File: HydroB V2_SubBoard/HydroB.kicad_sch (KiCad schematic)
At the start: 0 parts

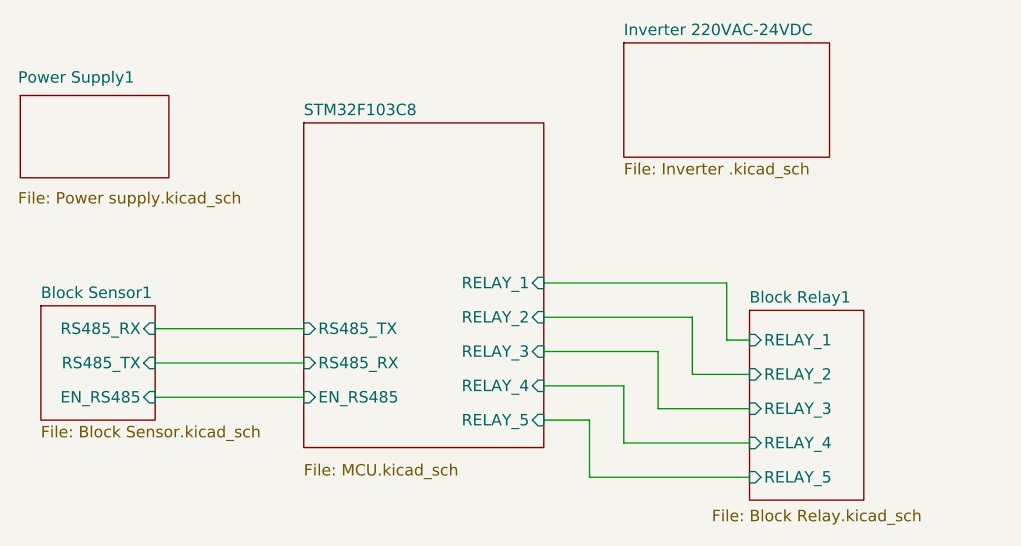
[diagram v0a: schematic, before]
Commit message: PCB update
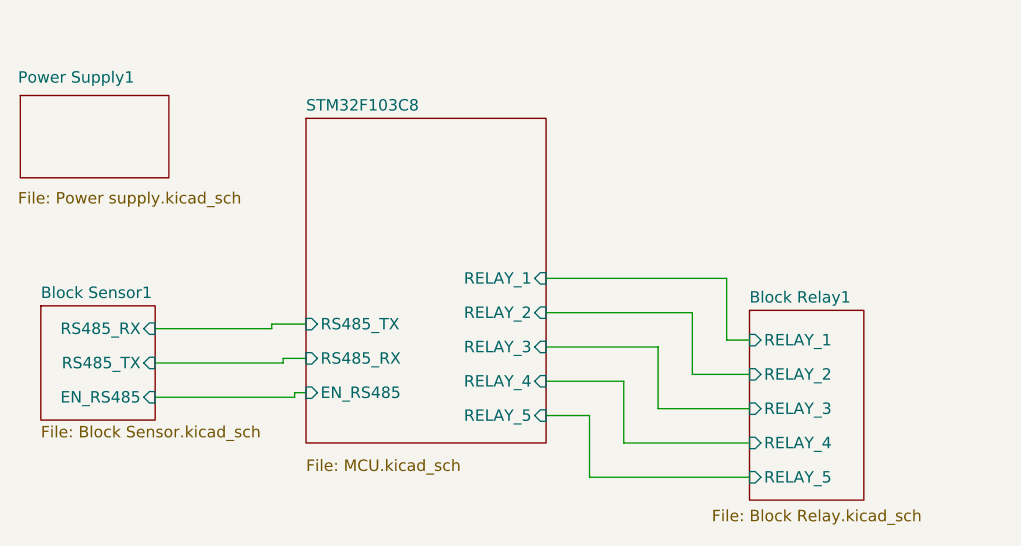
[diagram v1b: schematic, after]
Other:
- removed sheet Inverter 220VAC-24VDC
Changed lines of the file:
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@@
 	(wire
 		(pts
-			(xy 110.236 98.298) (xy 126.746 98.298)
+			(xy 123.19 97.79) (xy 127 97.79)
 		)
 		(stroke
@@
 	(wire
 		(pts
-			(xy 173.736 93.218) (xy 153.416 93.218)
+			(xy 173.736 92.71) (xy 153.67 92.71)
 		)
 		(stroke
@@
 	(wire
 		(pts
-			(xy 166.116 100.838) (xy 153.416 100.838)
-		)
-		(stroke
-			(width 0)
-			(type default)
-		)
-	)
-	(wire
-		(pts
-			(xy 158.496 108.458) (xy 153.416 108.458)
-		)
-		(stroke
-			(width 0)
-			(type default)
-		)
-	)
-	(wire
-		(pts
-			(xy 169.926 97.028) (xy 153.416 97.028)
+			(xy 166.116 100.33) (xy 153.67 100.33)
+		)
+		(stroke
+			(width 0)
+			(type default)
+		)
+	)
+	(wire
+		(pts
+			(xy 158.496 107.95) (xy 153.67 107.95)
+		)
+		(stroke
+			(width 0)
+			(type default)
+		)
+	)
+	(wire
+		(pts
+			(xy 123.19 97.79) (xy 123.19 98.298)
+		)
+		(stroke
+			(width 0)
+			(type default)
+		)
+	)
+	(wire
+		(pts
+			(xy 125.73 105.41) (xy 125.73 105.918)
+		)
+		(stroke
+			(width 0)
+			(type default)
+		)
+	)
+	(wire
+		(pts
+			(xy 124.46 101.6) (xy 124.46 102.108)
+		)
+		(stroke
+			(width 0)
+			(type default)
+		)
+	)
+	(wire
+		(pts
+			(xy 169.926 96.52) (xy 153.67 96.52)
+		)
+		(stroke
+			(width 0)
+			(type default)
+		)
+	)
+	(wire
+		(pts
+			(xy 125.73 105.918) (xy 110.236 105.918)
 		)
 		(stroke
@@
 	(wire
 		(pts
-			(xy 110.236 102.108) (xy 126.746 102.108)
+			(xy 124.46 101.6) (xy 127 101.6)
 		)
 		(stroke
@@
 	(wire
 		(pts
-			(xy 158.496 114.808) (xy 158.496 108.458)
-		)
-		(stroke
-			(width 0)
-			(type default)
-		)
-	)
-	(wire
-		(pts
-			(xy 110.236 105.918) (xy 126.746 105.918)
-		)
-		(stroke
-			(width 0)
-			(type default)
-		)
-	)
-	(wire
-		(pts
-			(xy 162.306 104.648) (xy 153.416 104.648)
-		)
-		(stroke
-			(width 0)
-			(type default)
-		)
-	)
-	(wire
-		(pts
-			(xy 169.926 103.378) (xy 169.926 97.028)
-		)
-		(stroke
-			(width 0)
-			(type default)
-		)
-	)
-	(wire
-		(pts
-			(xy 162.306 110.998) (xy 162.306 104.648)
-		)
-		(stroke
-			(width 0)
-			(type default)
-		)
-	)
-	(wire
-		(pts
-			(xy 166.116 107.188) (xy 166.116 100.838)
-		)
-		(stroke
-			(width 0)
-			(type default)
-		)
-	)
-	(wire
-		(pts
-			(xy 173.736 99.568) (xy 173.736 93.218)
+			(xy 158.496 114.808) (xy 158.496 107.95)
+		)
+		(stroke
+			(width 0)
+			(type default)
+		)
+	)
+	(wire
+		(pts
+			(xy 125.73 105.41) (xy 127 105.41)
+		)
+		(stroke
+			(width 0)
+			(type default)
+		)
+	)
+	(wire
+		(pts
+			(xy 162.306 104.14) (xy 153.67 104.14)
+		)
+		(stroke
+			(width 0)
+			(type default)
+		)
+	)
+	(wire
+		(pts
+			(xy 124.46 102.108) (xy 110.236 102.108)
+		)
+		(stroke
+			(width 0)
+			(type default)
+		)
+	)
+	(wire
+		(pts
+			(xy 169.926 103.378) (xy 169.926 96.52)
+		)
+		(stroke
+			(width 0)
+			(type default)
+		)
+	)
+	(wire
+		(pts
+			(xy 162.306 110.998) (xy 162.306 104.14)
+		)
+		(stroke
+			(width 0)
+			(type default)
+		)
+	)
+	(wire
+		(pts
+			(xy 123.19 98.298) (xy 110.236 98.298)
+		)
+		(stroke
+			(width 0)
+			(type default)
+		)
+	)
+	(wire
+		(pts
+			(xy 166.116 107.188) (xy 166.116 100.33)
+		)
+		(stroke
+			(width 0)
+			(type default)
+		)
+	)
+	(wire
+		(pts
+			(xy 173.736 99.568) (xy 173.736 92.71)
 		)
 		(stroke
@@
 	)
 	(sheet
-		(at 162.306 66.548)
-		(size 22.86 12.7)
-		(fields_autoplaced yes)
-		(stroke
-			(width 0.1524)
-			(type solid)
-		)
-		(fill
-			(color 221 133 0 1.0000)
-		)
-		(property "Sheetname" "Inverter 220VAC-24VDC"
-			(at 162.306 65.8364 0)
-			(effects
-				(font
-					(size 1.27 1.27)
-				)
-				(justify left bottom)
-			)
-		)
-		(property "Sheetfile" "Inverter .kicad_sch"
-			(at 162.306 79.8326 0)
-			(effects
-				(font
-					(size 1.27 1.27)
-				)
-				(justify left top)
-			)
-		)
-		(instances
-			(project "HydroB V2"
-				(path "/0a8bb8df-6bdd-4d10-933b-144d3fa4f517/b5cea501-254b-4c6a-af47-d8c013c279ab"
-					(page "8")
-				)
-			)
-		)
-	)
-	(sheet
 		(at 95.25 72.39)
 		(size 16.51 9.144)
@@
 	)
 	(sheet
-		(at 126.746 75.438)
+		(at 127 74.93)
 		(size 26.67 36.068)
 		(stroke
@@
 		)
 		(property "Sheetname" "STM32F103C8"
-			(at 126.746 74.7264 0)
+			(at 127 74.2184 0)
 			(effects
 				(font
@@
 		)
 		(property "Sheetfile" "MCU.kicad_sch"
-			(at 126.746 113.284 0)
+			(at 127 112.776 0)
 			(effects
 				(font
@@
 		)
 		(pin "RS485_RX" input
-			(at 126.746 102.108 180)
+			(at 127 101.6 180)
 			(effects
 				(font
@@
 		)
 		(pin "RS485_TX" input
-			(at 126.746 98.298 180)
+			(at 127 97.79 180)
 			(effects
 				(font
@@
 		)
 		(pin "EN_RS485" input
-			(at 126.746 105.918 180)
+			(at 127 105.41 180)
 			(effects
 				(font
@@
 		)
 		(pin "RELAY_5" input
-			(at 153.416 108.458 0)
+			(at 153.67 107.95 0)
 			(effects
 				(font
@@
 		)
 		(pin "RELAY_4" input
-			(at 153.416 104.648 0)
+			(at 153.67 104.14 0)
 			(effects
 				(font
@@
 		)
 		(pin "RELAY_2" input
-			(at 153.416 97.028 0)
+			(at 153.67 96.52 0)
 			(effects
 				(font
@@
 		)
 		(pin "RELAY_3" input
-			(at 153.416 100.838 0)
+			(at 153.67 100.33 0)
 			(effects
 				(font
@@
 		)
 		(pin "RELAY_1" input
-			(at 153.416 93.218 0)
-			(effects
-				(font
+			(at 153.67 92.71 0)
+			(effects
+				(font
